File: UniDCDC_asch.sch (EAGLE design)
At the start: 13 parts

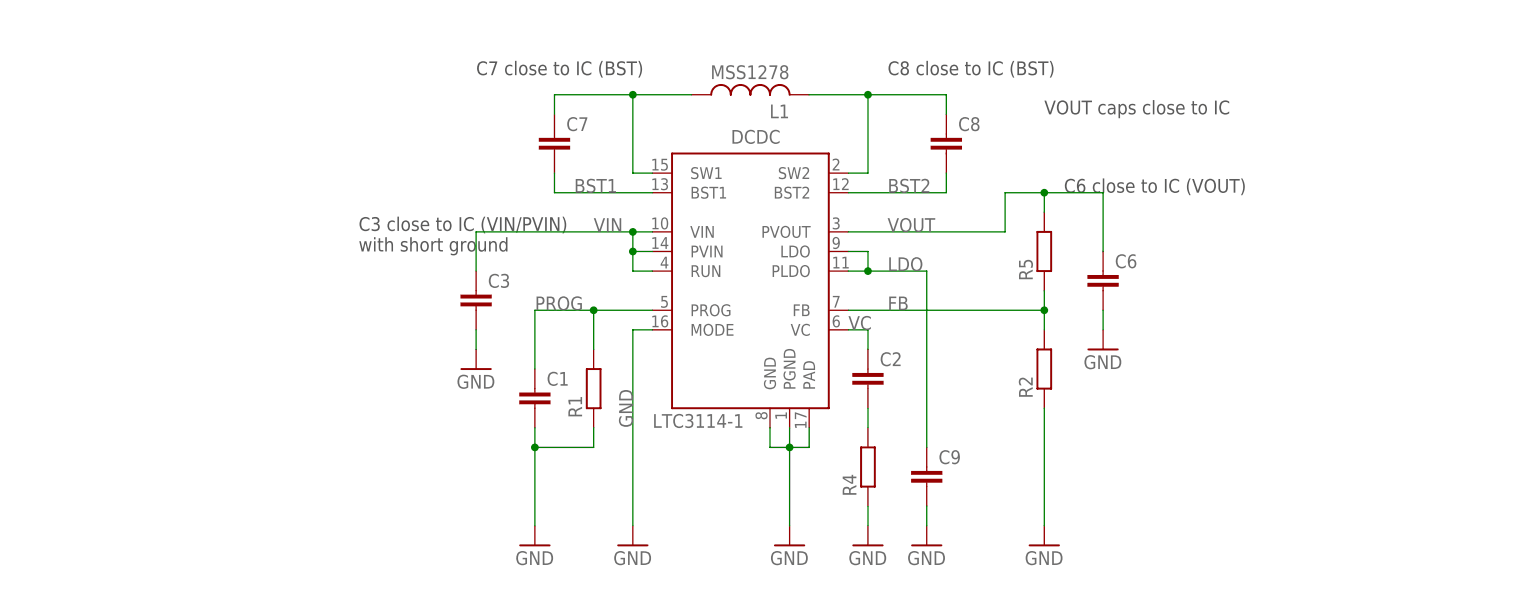
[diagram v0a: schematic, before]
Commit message: Manufacturing version
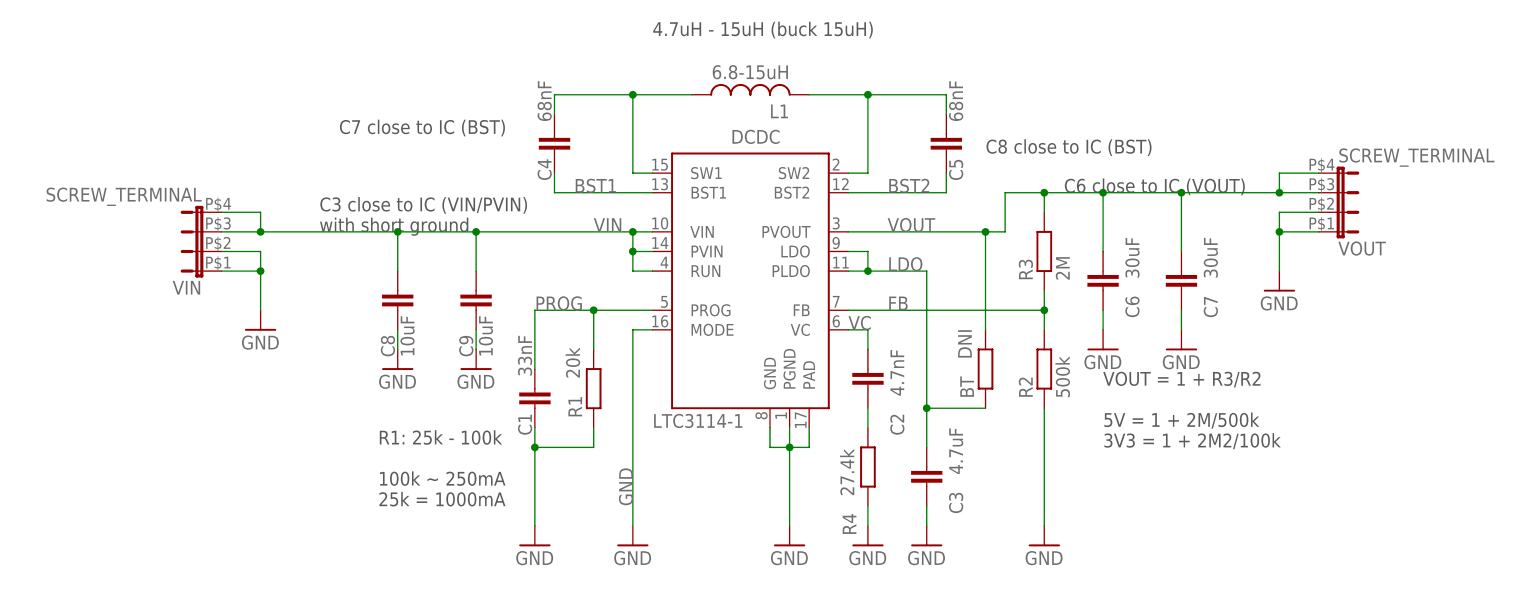
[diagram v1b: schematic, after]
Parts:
- added BT: DNI, rcl:R-EU_R0805
- added C4, C5: 68nF, rcl:C-EUC0805K
- added VIN, VOUT: SCREW_TERMINAL, uni_dcdc:SCREW_TERMINAL
- C1: value (none) -> 33nF
- C2: value (none) -> 4.7nF
- C3: value (none) -> 4.7uF
- C6, C7: value (none) -> 30uF
- C8, C9: value (none) -> 10uF
- L1: value MSS1278 -> 6.8-15uH
- R1: value (none) -> 20k
- R2: value (none) -> 500k
- R3: value (none) -> 2M
- R4: value (none) -> 27.4k
- renumbered R5 to R3
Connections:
- net BST1: now also C4.2; no longer C7.2
- net BST2: now also C5.2; no longer C8.2
- net GND: now also C7.2, C8.2, VIN.1, VIN.2, VOUT.1, VOUT.2
- net LDO: now also BT.1, C3.1; no longer C9.1
- net N$11: now also C4.1; no longer C7.1
- net N$12: now also C5.1; no longer C8.1
- net VIN: now also C8.1, C9.1, VIN.3, VIN.4; no longer C3.1
- net VOUT: now also BT.2, C7.1, VOUT.3, VOUT.4
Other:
- note added: "4.7uH - 15uH (buck 15uH)"
- note added: "R1: 25k - 100k 100k ~ 250mA 25k = 1000mA"
- note added: "VOUT = 1 + R3/R2 5V = 1 + 2M/500k 3V3 = 1 + 2M2/100k"
- note removed: "VOUT caps close to IC"
- moved on the sheet: C3, C7, C8, C9
